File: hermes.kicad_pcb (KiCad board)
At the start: 2 copper layers, 48.5 x 45.5 mm, 7 parts, among them J1 OLED Header, U1 XIAO RP2040, U2 LSM6DS3TR-C

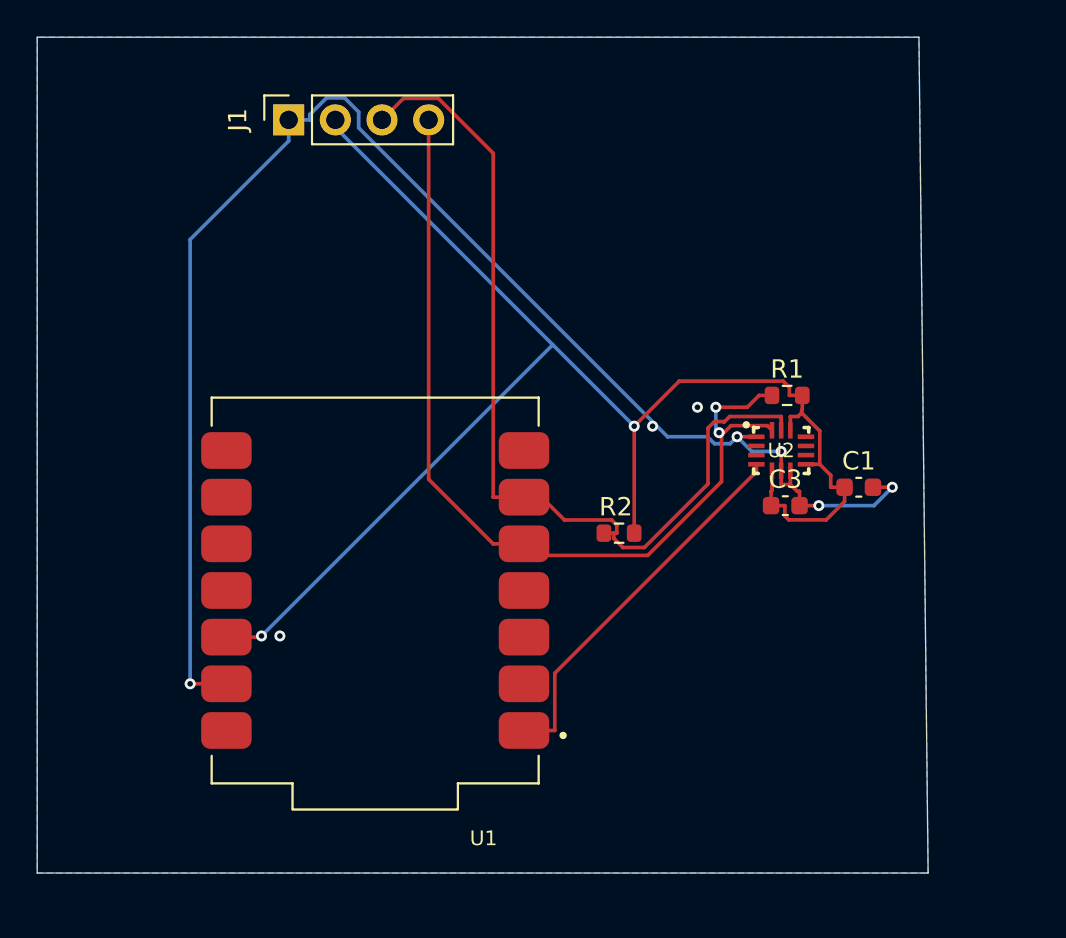
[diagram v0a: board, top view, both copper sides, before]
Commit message: Add files via upload
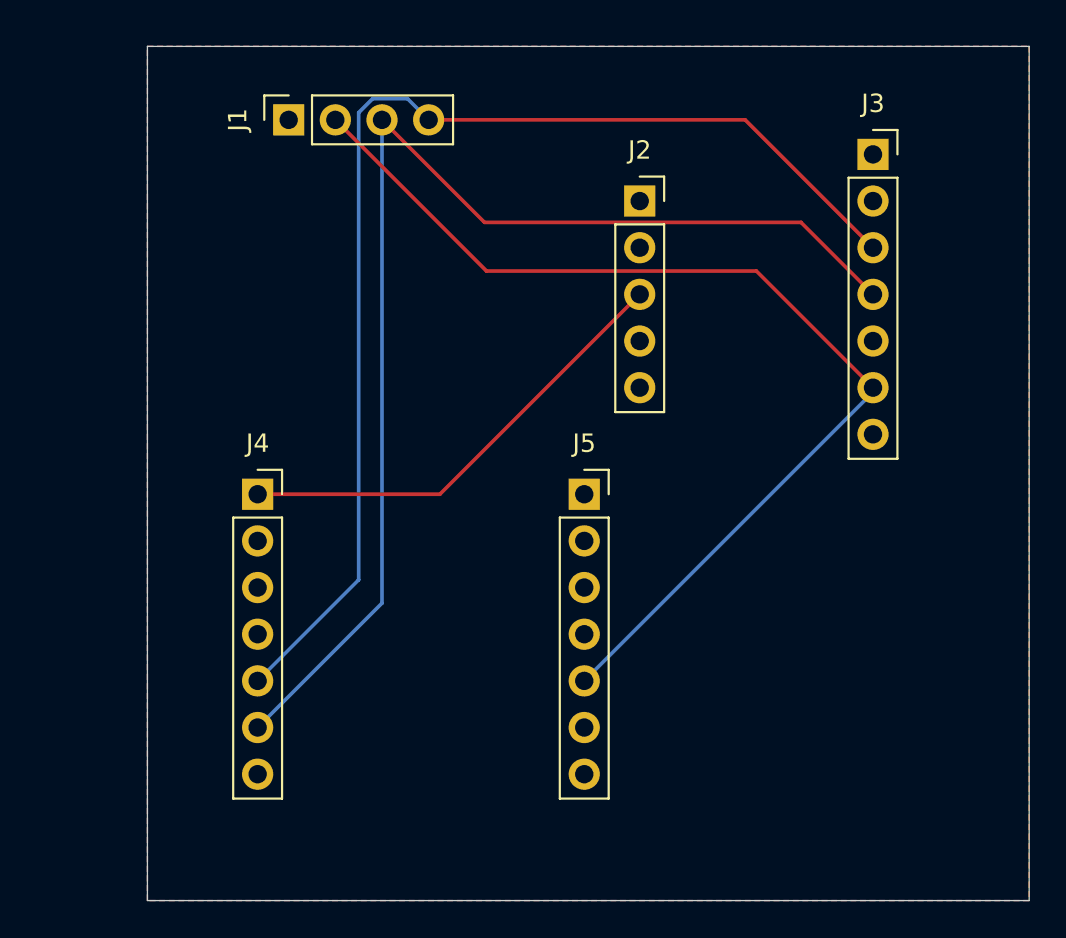
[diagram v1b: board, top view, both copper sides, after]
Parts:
- removed C1, C3: 0.1uF, Capacitor_SMD:C_0603_1608Metric
- removed R1, R2: 4.7k, Resistor_SMD:R_0603_1608Metric
- removed U1: XIAO RP2040, 67:MODULE_102010428
- removed U2: LSM6DS3TR-C, 67:LGA-14-2.5X3MM
- added J2: sensor header 2, Connector_PinSocket_2.54mm:PinSocket_1x05_P2.54mm_Vertical, F.Cu at (137.3, 80.4)
- added J3: sensor header 1, Connector_PinSocket_2.54mm:PinSocket_1x07_P2.54mm_Vertical, F.Cu at (150.0, 77.9)
- added J4: XIAO header 1, Connector_PinSocket_2.54mm:PinSocket_1x07_P2.54mm_Vertical, F.Cu at (116.5, 96.4)
- added J5: XIAO header 2, Connector_PinSocket_2.54mm:PinSocket_1x07_P2.54mm_Vertical, F.Cu at (134.3, 96.4)
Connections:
- J1 pad 2: /<NO NET> -> /3V3
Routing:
- net GND: track 83.2 -> 0.00 mm, vias 8 -> 0
- net /<NO NET>: track 80.7 -> 0.00 mm, vias 2 -> 0
- net /3V3: track 0.00 -> 57.8 mm
- net /SCL: track 50.1 -> 66.5 mm
- net /SDA: track 49.5 -> 64.9 mm, vias 2 -> 0
- net /INT: track 20.7 -> 25.3 mm
- added copper zone on F.Cu, net GND
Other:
- board size 48.5 x 45.5 mm -> 48 x 46.5 mm
